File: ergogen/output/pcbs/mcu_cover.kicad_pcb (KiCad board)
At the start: 2 copper layers, 20.5 x 58 mm, 2 parts

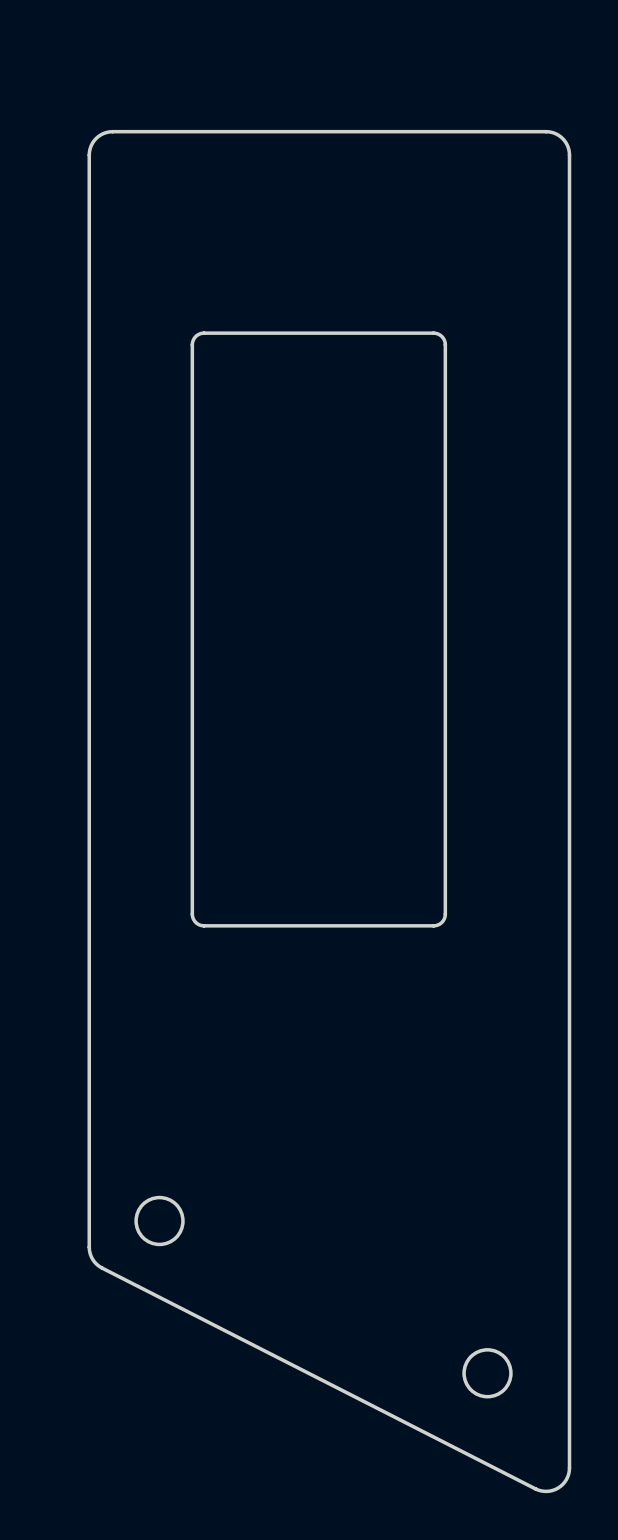
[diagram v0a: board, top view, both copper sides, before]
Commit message: new shape
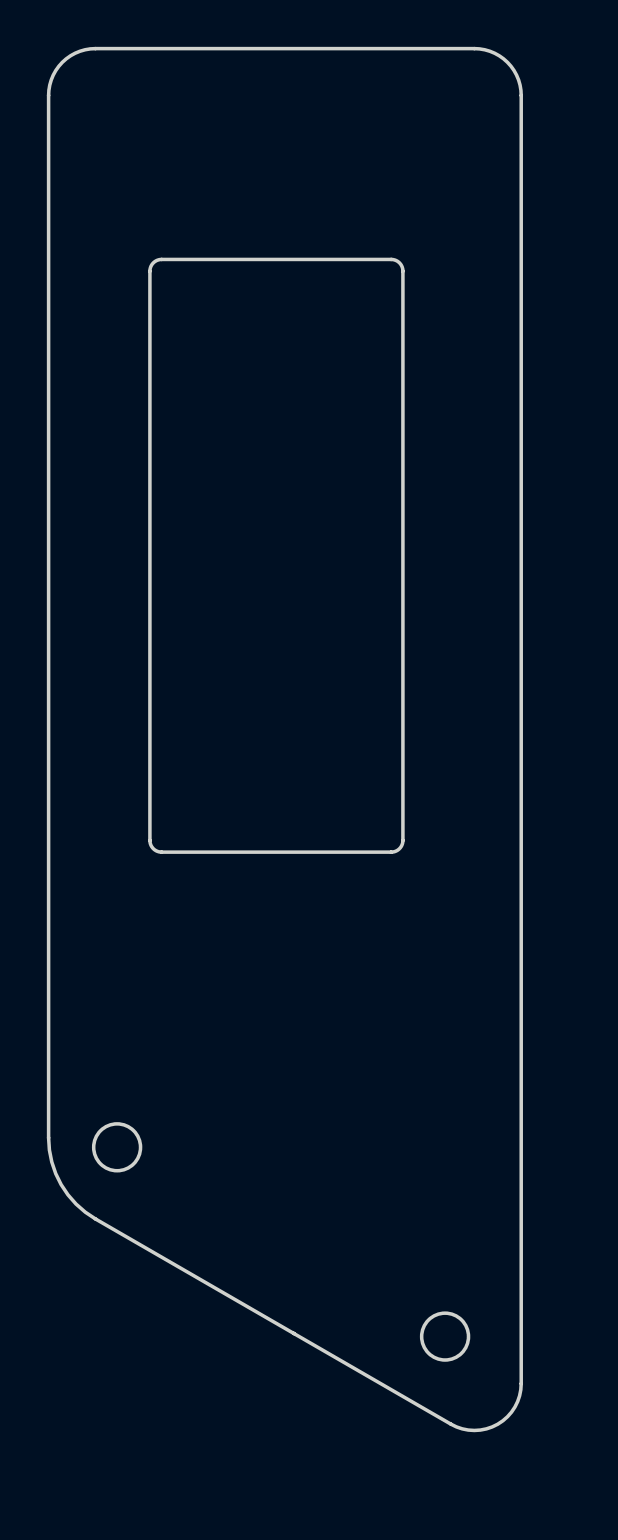
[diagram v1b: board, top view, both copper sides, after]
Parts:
- moved MH1 3.63 mm to (149.5, 86.4)
- moved MH2 2.39 mm to (163.5, 94.5)
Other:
- board size 20.5 x 58 mm -> 20.2 x 59 mm
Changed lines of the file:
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@@
   (title_block
     (title "mcu_cover")
-    (date "2025-11-02")
+    (date "2025-11-10")
     (rev "1")
     (company "curtis bollinger")
@@
   (footprint "ceoloide:mounting_hole_npth"
     (layer "F.Cu")
-    (at 151.2922031 89.53066630000001 0)
+    (at 149.48162050000002 86.38459739999999 0)
     (property "Reference" "MH1"
       (at 0 2.55 0)
@@
   (footprint "ceoloide:mounting_hole_npth"
     (layer "F.Cu")
-    (at 165.2922031 96.03066630000001 0)
+    (at 163.48162050000002 94.46459739999999 0)
     (property "Reference" "MH2"
       (at 0 2.55 0)
@@
     )
   )
-  (gr_line (start 168.7922031 100.07308144572157) (end 168.7922031 44.03066630000001) (layer Edge.Cuts) (stroke (width 0.15) (type default)))
-(gr_line (start 167.7922031 43.03066630000001) (end 149.2922031 43.03066630000001) (layer Edge.Cuts) (stroke (width 0.15) (type default)))
-(gr_line (start 148.2922031 90.64686063325334) (end 148.2922031 44.03066630000001) (layer Edge.Cuts) (stroke (width 0.15) (type default)))
-(gr_line (start 148.8382126 91.53786713325334) (end 167.33821260000002 100.96408794572159) (layer Edge.Cuts) (stroke (width 0.15) (type default)))
-(gr_line (start 153.1922031 76.93066630000001) (end 162.9922031 76.93066630000001) (layer Edge.Cuts) (stroke (width 0.15) (type default)))
-(gr_line (start 163.4922031 76.43066630000001) (end 163.4922031 52.130666300000016) (layer Edge.Cuts) (stroke (width 0.15) (type default)))
-(gr_line (start 162.9922031 51.630666300000016) (end 153.1922031 51.630666300000016) (layer Edge.Cuts) (stroke (width 0.15) (type default)))
-(gr_line (start 152.6922031 52.130666300000016) (end 152.6922031 76.43066630000001) (layer Edge.Cuts) (stroke (width 0.15) (type default)))
-(gr_arc (start 162.9922031 76.93066630000001) (mid 163.34575650000002 76.78421970000001) (end 163.4922031 76.43066630000001) (layer Edge.Cuts) (stroke (width 0.15) (type default)))
-(gr_arc (start 163.4922031 52.130666300000016) (mid 163.34575650000002 51.77711290000001) (end 162.9922031 51.630666300000016) (layer Edge.Cuts) (stroke (width 0.15) (type default)))
-(gr_arc (start 153.1922031 51.630666300000016) (mid 152.8386497 51.77711290000001) (end 152.6922031 52.130666300000016) (layer Edge.Cuts) (stroke (width 0.15) (type default)))
-(gr_arc (start 152.6922031 76.43066630000001) (mid 152.8386497 76.78421970000001) (end 153.1922031 76.93066630000001) (layer Edge.Cuts) (stroke (width 0.15) (type default)))
-(gr_arc (start 168.7922031 44.03066630000001) (mid 168.4993099 43.32355950000001) (end 167.7922031 43.03066630000001) (layer Edge.Cuts) (stroke (width 0.15) (type default)))
-(gr_arc (start 149.2922031 43.03066630000001) (mid 148.5850963 43.32355950000001) (end 148.2922031 44.03066630000001) (layer Edge.Cuts) (stroke (width 0.15) (type default)))
-(gr_arc (start 148.2922031 90.64686063325334) (mid 148.4395629 91.16935923325335) (end 148.8382126 91.53786713325334) (layer Edge.Cuts) (stroke (width 0.15) (type default)))
-(gr_arc (start 167.3382126 100.96408794572157) (mid 168.3147016 100.92572154572157) (end 168.7922031 100.07308144572157) (layer Edge.Cuts) (stroke (width 0.15) (type default)))
-(gr_circle (center 151.2922031 89.53066630000001) (end 152.2922031 89.53066630000001) (layer Edge.Cuts) (stroke (width 0.15) (type default)) (fill none))
-(gr_circle (center 165.2922031 96.03066630000001) (end 166.2922031 96.03066630000001) (layer Edge.Cuts) (stroke (width 0.15) (type default)) (fill none))
+  (gr_line (start 166.73162050017376 96.47131793428673) (end 166.73162050017376 41.4845974) (layer Edge.Cuts) (stroke (width 0.15) (type default)))
+(gr_line (start 164.73162050017376 39.4845974) (end 148.55712050000002 39.4845974) (layer Edge.Cuts) (stroke (width 0.15) (type default)))
+(gr_line (start 146.55712050000002 85.97848666737389) (end 146.55712050000002 41.4845974) (layer Edge.Cuts) (stroke (width 0.15) (type default)))
+(gr_line (start 148.55712050000005 89.44258826737392) (end 157.02419341559587 94.33105510345534) (layer Edge.Cuts) (stroke (width 0.15) (type default)))
+(gr_arc (start 146.55712050000002 85.97848666737389) (mid 147.09301890000003 87.97848666737389) (end 148.55712050000002 89.44258826737389) (layer Edge.Cuts) (stroke (width 0.15) (type default)))
+(gr_line (start 163.73162050017373 98.20336873428671) (end 157.0242892 94.33088919999997) (layer Edge.Cuts) (stroke (width 0.15) (type default)))
+(gr_line (start 157.0242892 94.33088919999997) (end 157.02419341559587 94.33105510345536) (layer Edge.Cuts) (stroke (width 0.15) (type default)))
+(gr_line (start 151.38162050000003 73.7845974) (end 161.18162050000004 73.7845974) (layer Edge.Cuts) (stroke (width 0.15) (type default)))
+(gr_line (start 161.68162050000004 73.2845974) (end 161.68162050000004 48.9845974) (layer Edge.Cuts) (stroke (width 0.15) (type default)))
+(gr_line (start 161.18162050000004 48.4845974) (end 151.38162050000003 48.4845974) (layer Edge.Cuts) (stroke (width 0.15) (type default)))
+(gr_line (start 150.88162050000003 48.9845974) (end 150.88162050000003 73.2845974) (layer Edge.Cuts) (stroke (width 0.15) (type default)))
+(gr_arc (start 161.18162050000004 73.7845974) (mid 161.53517390000005 73.63815079999999) (end 161.68162050000004 73.2845974) (layer Edge.Cuts) (stroke (width 0.15) (type default)))
+(gr_arc (start 161.68162050000004 48.9845974) (mid 161.53517390000005 48.631043999999996) (end 161.18162050000004 48.4845974) (layer Edge.Cuts) (stroke (width 0.15) (type default)))
+(gr_arc (start 151.38162050000003 48.4845974) (mid 151.02806710000002 48.631043999999996) (end 150.88162050000003 48.9845974) (layer Edge.Cuts) (stroke (width 0.15) (type default)))
+(gr_arc (start 150.88162050000003 73.2845974) (mid 151.02806710000002 73.63815079999999) (end 151.38162050000003 73.7845974) (layer Edge.Cuts) (stroke (width 0.15) (type default)))
+(gr_arc (start 166.73162050017376 41.4845974) (mid 166.14583410017377 40.0703838) (end 164.73162050017376 39.4845974) (layer Edge.Cuts) (stroke (width 0.15) (type default)))
+(gr_arc (start 148.55712050000002 39.4845974) (mid 147.1429069 40.0703838) (end 146.55712050000002 41.4845974) (layer Edge.Cuts) (stroke (width 0.15) (type default)))
+(gr_arc (start 163.73162050017376 98.20336873428673) (mid 165.73162050017376 98.20336873428673) (end 166.73162050017376 96.47131793428673) (layer Edge.Cuts) (stroke (width 0.15) (type default)))
+(gr_circle (center 149.48162050000002 86.38459739999999) (end 150.48162050000002 86.38459739999999) (layer Edge.Cuts) (stroke (width 0.15) (type default)) (fill none))
+(gr_circle (center 163.48162050000002 94.46459739999999) (end 164.48162050000002 94.46459739999999) (layer Edge.Cuts) (stroke (width 0.15) (type default)) (fill none))
 )

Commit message: update generated files
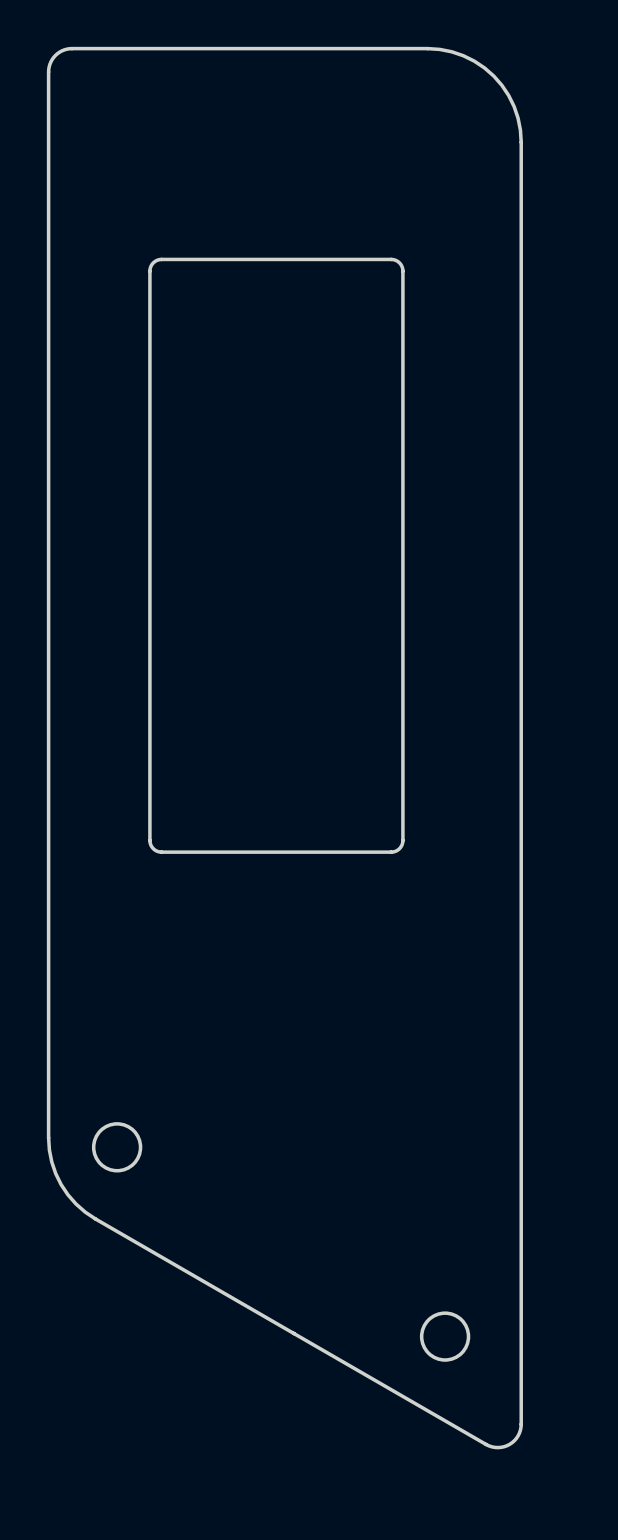
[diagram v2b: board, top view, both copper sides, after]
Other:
- board size 20.2 x 59 mm -> 20.2 x 59.7 mm
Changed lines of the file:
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@@
   (title_block
     (title "mcu_cover")
-    (date "2025-11-10")
+    (date "2025-11-12")
     (rev "1")
     (company "curtis bollinger")
@@
     )
   )
-  (gr_line (start 166.73162050017376 96.47131793428673) (end 166.73162050017376 41.4845974) (layer Edge.Cuts) (stroke (width 0.15) (type default)))
-(gr_line (start 164.73162050017376 39.4845974) (end 148.55712050000002 39.4845974) (layer Edge.Cuts) (stroke (width 0.15) (type default)))
-(gr_line (start 146.55712050000002 85.97848666737389) (end 146.55712050000002 41.4845974) (layer Edge.Cuts) (stroke (width 0.15) (type default)))
+  (gr_line (start 166.73162050017376 98.20336873864981) (end 166.73162050000002 43.4845974) (layer Edge.Cuts) (stroke (width 0.15) (type default)))
+(gr_line (start 147.55712050000002 39.4845974) (end 162.73162050000002 39.4845974) (layer Edge.Cuts) (stroke (width 0.15) (type default)))
+(gr_arc (start 166.73162050000002 43.4845974) (mid 165.56004760000002 40.6561703) (end 162.73162050000002 39.4845974) (layer Edge.Cuts) (stroke (width 0.15) (type default)))
+(gr_line (start 146.55712050000002 85.97848666737389) (end 146.55712050000002 40.4845974) (layer Edge.Cuts) (stroke (width 0.15) (type default)))
 (gr_line (start 148.55712050000005 89.44258826737392) (end 157.02419341559587 94.33105510345534) (layer Edge.Cuts) (stroke (width 0.15) (type default)))
 (gr_arc (start 146.55712050000002 85.97848666737389) (mid 147.09301890000003 87.97848666737389) (end 148.55712050000002 89.44258826737389) (layer Edge.Cuts) (stroke (width 0.15) (type default)))
-(gr_line (start 163.73162050017373 98.20336873428671) (end 157.0242892 94.33088919999997) (layer Edge.Cuts) (stroke (width 0.15) (type default)))
+(gr_line (start 165.23162050017376 99.06939413864981) (end 157.0242892 94.33088919999997) (layer Edge.Cuts) (stroke (width 0.15) (type default)))
 (gr_line (start 157.0242892 94.33088919999997) (end 157.02419341559587 94.33105510345536) (layer Edge.Cuts) (stroke (width 0.15) (type default)))
 (gr_line (start 151.38162050000003 73.7845974) (end 161.18162050000004 73.7845974) (layer Edge.Cuts) (stroke (width 0.15) (type default)))
@@
 (gr_arc (start 151.38162050000003 48.4845974) (mid 151.02806710000002 48.631043999999996) (end 150.88162050000003 48.9845974) (layer Edge.Cuts) (stroke (width 0.15) (type default)))
 (gr_arc (start 150.88162050000003 73.2845974) (mid 151.02806710000002 73.63815079999999) (end 151.38162050000003 73.7845974) (layer Edge.Cuts) (stroke (width 0.15) (type default)))
-(gr_arc (start 166.73162050017376 41.4845974) (mid 166.14583410017377 40.0703838) (end 164.73162050017376 39.4845974) (layer Edge.Cuts) (stroke (width 0.15) (type default)))
-(gr_arc (start 148.55712050000002 39.4845974) (mid 147.1429069 40.0703838) (end 146.55712050000002 41.4845974) (layer Edge.Cuts) (stroke (width 0.15) (type default)))
-(gr_arc (start 163.73162050017376 98.20336873428673) (mid 165.73162050017376 98.20336873428673) (end 166.73162050017376 96.47131793428673) (layer Edge.Cuts) (stroke (width 0.15) (type default)))
+(gr_arc (start 147.55712050000002 39.4845974) (mid 146.85001370000003 39.7774906) (end 146.55712050000002 40.4845974) (layer Edge.Cuts) (stroke (width 0.15) (type default)))
+(gr_arc (start 165.23162050017376 99.06939413864981) (mid 166.23162050017376 99.06939413864981) (end 166.73162050017376 98.20336873864981) (layer Edge.Cuts) (stroke (width 0.15) (type default)))
 (gr_circle (center 149.48162050000002 86.38459739999999) (end 150.48162050000002 86.38459739999999) (layer Edge.Cuts) (stroke (width 0.15) (type default)) (fill none))
 (gr_circle (center 163.48162050000002 94.46459739999999) (end 164.48162050000002 94.46459739999999) (layer Edge.Cuts) (stroke (width 0.15) (type default)) (fill none))
